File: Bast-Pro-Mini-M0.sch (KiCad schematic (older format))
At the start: 18 parts, among them J1 USB_B_Micro, J2 Conn_02x02_Odd_Even, P1 Digital, P2 ADC, P3 Analog, SW1 SW_DPST_x2, U1 AP2112K-3.3TRG1, U2 ATSAMD21E18A-AF

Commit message: Add BOM
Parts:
- C1: manf# (none) -> 885012106022
- C2: manf# (none) -> 885012106011
- C3, C4, C5: manf# (none) -> 885012206071
- D1: manf# (none) -> AP2012EC
- D2: manf# (none) -> APT2012SGC
- F1: manf# (none) -> MFU0805FF00500P100
- J1: manf# (none) -> 629105150521
- R1, R2: manf# (none) -> ESR03EZPJ331
- SW1: manf# (none) -> B3U-1000P-B
- U1: symbol Croketa-cache:AP2112K-3.3TRG1 -> Bast-Pro-Mini-M0-rescue:AP2112K-3.3TRG1-Croketa-cache; Campo4 Diodes Inc. -> (none); Campo5 SOT-753 Diodes Inc. -> (none); Campo6 None -> (none); Campo7 Unavailable -> (none); Campo8 AP2112 Series 0.6 A 3.3 V Fixed Output SMT LDO Linear Regul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 -> (none); manf# (none) -> AP2112K-3.3TRG1
- U2: symbol Croketa-cache:ATSAMD21E18A-AF -> Bast-Pro-Mini-M0-rescue:ATSAMD21E18A-AF-Croketa-cache; Campo4 Microchip -> (none); Campo5 TQFP-32 Microchip -> (none); Campo6 3.12 USD -> (none); Campo7 Good -> (none); Campo8 MCU 32-Bit SAM D21E ARM Cortex M0+ RISC 256KB Flash 3.3V 32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 -> (none); manf# (none) -> ATSAMD21E18A-AU
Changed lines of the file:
@@
 Sheet 1 1
 Title "Bast Pro Mini M0"
-Date "2018-10-08"
+Date "2019-01-10"
 Rev "0.2"
 Comp "Electronic Cats"
 Comment1 "Edgar Capuchino"
 Comment2 "Andrés Sabas"
-Comment3 ""
+Comment3 "Eduardo Contreras"
 Comment4 ""
 $EndDescr
@@
 1
 $Comp
-L Croketa-cache:ATSAMD21E18A-AF U2
+L Bast-Pro-Mini-M0-rescue:ATSAMD21E18A-AF-Croketa-cache U2
 U 1 1 5BAEC202
 P 5030 2010
@@
 F 2 "Package_QFP:TQFP-32_7x7mm_P0.8mm" H 5030 2010 50  0001 L BNN
 F 3 "ATSAMD21E18A-AF" H 5030 2010 50  0001 L BNN
-F 4 "Microchip" H 5030 2010 50  0001 L BNN "Campo4"
-F 5 "TQFP-32 Microchip" H 5030 2010 50  0001 L BNN "Campo5"
-F 6 "3.12 USD" H 5030 2010 50  0001 L BNN "Campo6"
-F 7 "Good" H 5030 2010 50  0001 L BNN "Campo7"
-F 8 "MCU 32-Bit SAM D21E ARM Cortex M0+ RISC 256KB Flash 3.3V 32-Pin TQFP Tray" H 5030 2010 50  0001 L BNN "Campo8"
+F 4 "ATSAMD21E18A-AU" H 5030 2010 50  0001 C CNN "manf#"
 	1    5030 2010
 	1    0    0    -1
@@
 F 2 "Capacitor_SMD:C_0603_1608Metric_Pad1.05x0.95mm_HandSolder" H 7180 1120 50  0001 C CNN
 F 3 "~" H 7180 1120 50  0001 C CNN
+F 4 "885012206071" H 7180 1120 50  0001 C CNN "manf#"
 	1    7180 1120
 	1    0    0    -1
@@
 F 2 "Capacitor_SMD:C_0603_1608Metric_Pad1.05x0.95mm_HandSolder" H 6940 1240 50  0001 C CNN
 F 3 "~" H 6940 1240 50  0001 C CNN
+F 4 "885012206071" H 6940 1240 50  0001 C CNN "manf#"
 	1    6940 1240
 	1    0    0    -1
@@
 F 2 "Capacitor_SMD:C_0603_1608Metric_Pad1.05x0.95mm_HandSolder" H 6680 1760 50  0001 C CNN
 F 3 "~" H 6680 1760 50  0001 C CNN
+F 4 "885012206071" H 6680 1760 50  0001 C CNN "manf#"
 	1    6680 1760
 	1    0    0    -1
@@
 F 2 "LED_SMD:LED_0805_2012Metric_Pad1.15x1.40mm_HandSolder" H 8560 1655 50  0001 C CNN
 F 3 "~" H 8560 1655 50  0001 C CNN
+F 4 "AP2012EC" V 8560 1655 50  0001 C CNN "manf#"
 	1    8560 1655
 	0    -1   -1   0
@@
 F 2 "LED_SMD:LED_0805_2012Metric_Pad1.15x1.40mm_HandSolder" H 9180 1655 50  0001 C CNN
 F 3 "~" H 9180 1655 50  0001 C CNN
+F 4 "APT2012SGC" V 9180 1655 50  0001 C CNN "manf#"
 	1    9180 1655
 	0    -1   -1   0
@@
 F 2 "Resistor_SMD:R_0603_1608Metric_Pad1.05x0.95mm_HandSolder" V 8490 2075 50  0001 C CNN
 F 3 "~" H 8560 2075 50  0001 C CNN
+F 4 "ESR03EZPJ331" H 8560 2075 50  0001 C CNN "manf#"
 	1    8560 2075
 	1    0    0    -1
@@
 F 2 "Resistor_SMD:R_0603_1608Metric_Pad1.05x0.95mm_HandSolder" V 9110 2085 50  0001 C CNN
 F 3 "~" H 9180 2085 50  0001 C CNN
+F 4 "ESR03EZPJ331" H 9180 2085 50  0001 C CNN "manf#"
 	1    9180 2085
 	1    0    0    -1
@@
 F 2 "Connector_USB:USB_Micro-B_Wuerth_629105150521" H 1400 4350 50  0001 C CNN
 F 3 "~" H 1400 4350 50  0001 C CNN
+F 4 "629105150521" H 1250 4400 50  0001 C CNN "manf#"
 	1    1250 4400
 	1    0    0    -1
@@
 F 2 "Fuse:Fuse_0805_2012Metric_Pad1.15x1.40mm_HandSolder" H 1960 4000 50  0001 L CNN
 F 3 "~" H 1910 4200 50  0001 C CNN
+F 4 "MFU0805FF00500P100" V 1910 4200 50  0001 C CNN "manf#"
 	1    1910 4200
 	0    1    1    0
@@
 F 2 "Capacitor_SMD:C_0603_1608Metric_Pad1.05x0.95mm_HandSolder" H 8010 4850 50  0001 C CNN
 F 3 "~" H 8010 4850 50  0001 C CNN
+F 4 "885012106022" H 8010 4850 50  0001 C CNN "manf#"
 	1    8010 4850
 	1    0    0    -1
 $EndComp
 $Comp
-L Croketa-cache:AP2112K-3.3TRG1 U1
+L Bast-Pro-Mini-M0-rescue:AP2112K-3.3TRG1-Croketa-cache U1
 U 1 1 5BB540C8
 P 9060 4720
@@
 F 2 "Package_TO_SOT_SMD:SOT-23-5" H 9060 4720 50  0001 L BNN
 F 3 "AP2112K-3.3TRG1" H 9060 4720 50  0001 L BNN
-F 4 "Diodes Inc." H 9060 4720 50  0001 L BNN "Campo4"
-F 5 "SOT-753 Diodes Inc." H 9060 4720 50  0001 L BNN "Campo5"
-F 6 "None" H 9060 4720 50  0001 L BNN "Campo6"
-F 7 "Unavailable" H 9060 4720 50  0001 L BNN "Campo7"
-F 8 "AP2112 Series 0.6 A 3.3 V Fixed Output SMT LDO Linear Regulator - SOT23-5" H 9060 4720 50  0001 L BNN "Campo8"
+F 4 "AP2112K-3.3TRG1" H 9060 4720 50  0001 C CNN "manf#"
 	1    9060 4720
 	1    0    0    -1
@@
 F 2 "Capacitor_SMD:C_0603_1608Metric_Pad1.05x0.95mm_HandSolder" H 10150 4670 50  0001 C CNN
 F 3 "~" H 10150 4670 50  0001 C CNN
+F 4 "885012106011" H 10150 4670 50  0001 C CNN "manf#"
 	1    10150 4670
 	1    0    0    -1
@@
 F 2 "Button_Switch_SMD:SW_SPST_B3U-1000P-B" H 10145 1730 50  0001 C CNN
 F 3 "" H 10145 1730 50  0001 C CNN
+F 4 "B3U-1000P-B" H 10145 1730 50  0001 C CNN "manf#"
 	1    10145 1730
 	1    0    0    -1
@@
 LED
 $Comp
-L Croketa-cache:+3.3V #PWR0101
+L Bast-Pro-Mini-M0-rescue:+3.3V-Croketa-cache #PWR0101
 U 1 1 5BBD0E40
 P 2630 1170

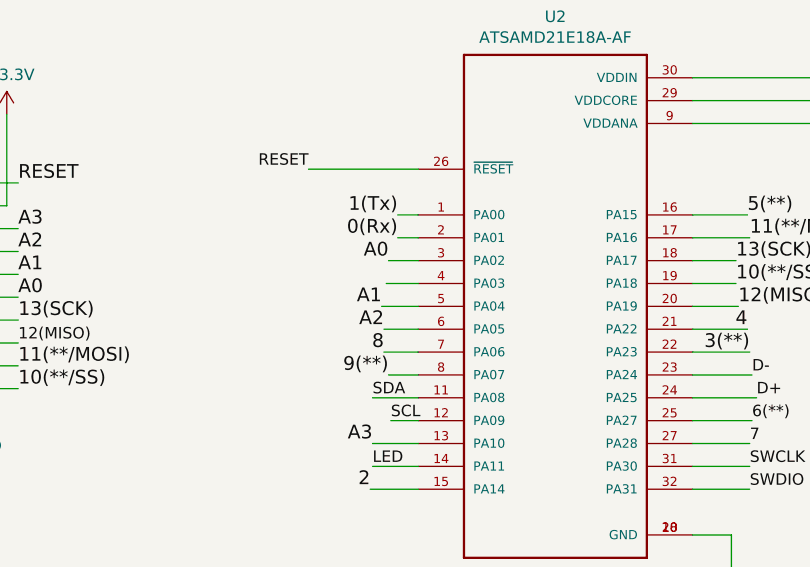
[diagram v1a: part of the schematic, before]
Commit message: bump :)
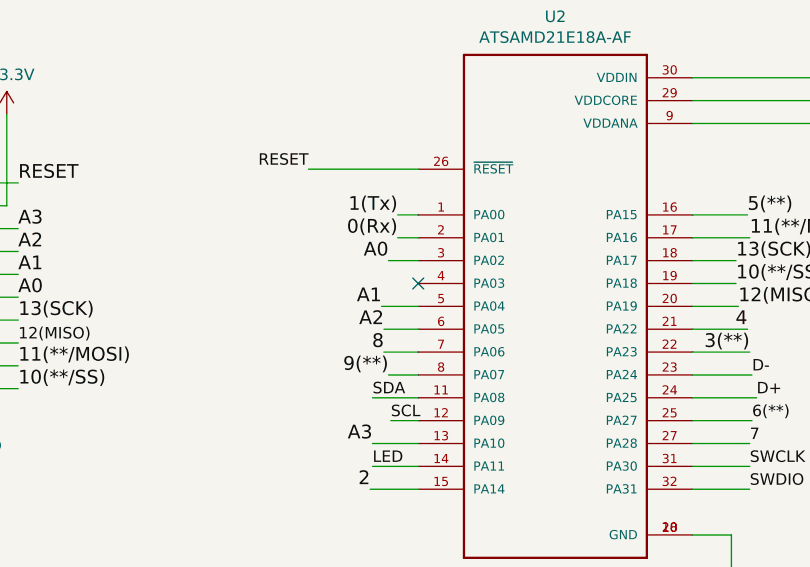
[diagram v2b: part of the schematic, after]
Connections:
- no-connect marks 1 -> 2
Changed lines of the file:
@@
 Wire Wire Line
 	4300 1810 4430 1810
-Wire Wire Line
-	4290 1910 4430 1910
 Text Label 4270 2010 2    60   ~ 0
 A1
@@
 Wire Wire Line
 	2530 1220 2530 1170
+NoConn ~ 4430 1910
 $EndSCHEMATC
